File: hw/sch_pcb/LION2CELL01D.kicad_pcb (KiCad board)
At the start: 2 copper layers, 80.8 x 60.5 mm, 100 parts, among them J1 JUMP_4X2, J10 JUMP_2x1, J11 JUMP_2x1, J12 JUMP_2x1, J13 JUMP_4X2, J14 JUMP_2x1, J15 CONN_2, J2 JUMP_2x1, J3 JUMP_2x1, J4 JUMP2_2x1, J5 JUMP_2x1, J6 JUMP_2x1, J7 JUMP_4X2, J8 CONN1_1, J9 CONN1_1, P1 _, P2 _, P3 _, P4 _, Q1 IRLML6244, SW1 SW_PUSH, U1 BQ29209, U2 BQ24103, U3 BQ34Z100, U4 SN74HC164D, U5 TPS76601, U6 APX810-31SAG-7

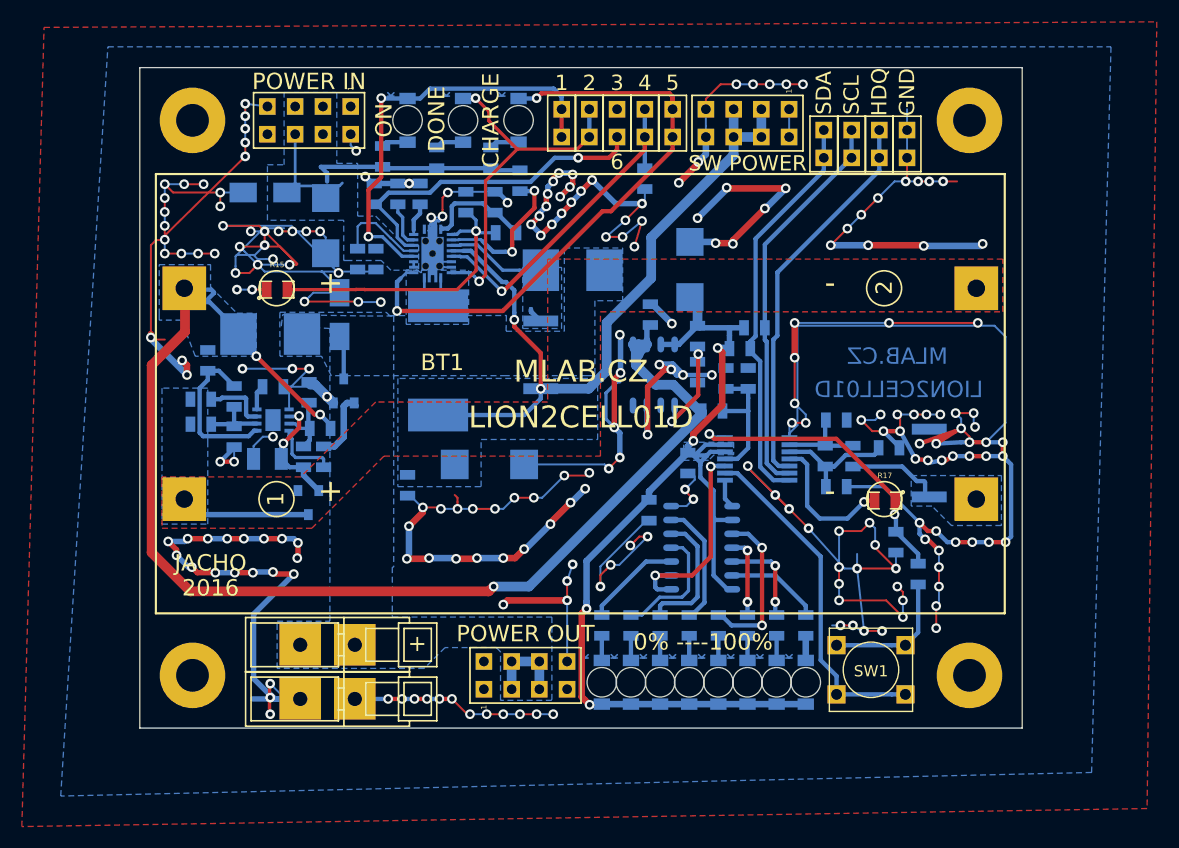
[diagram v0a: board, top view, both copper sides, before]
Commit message: Documentation update.
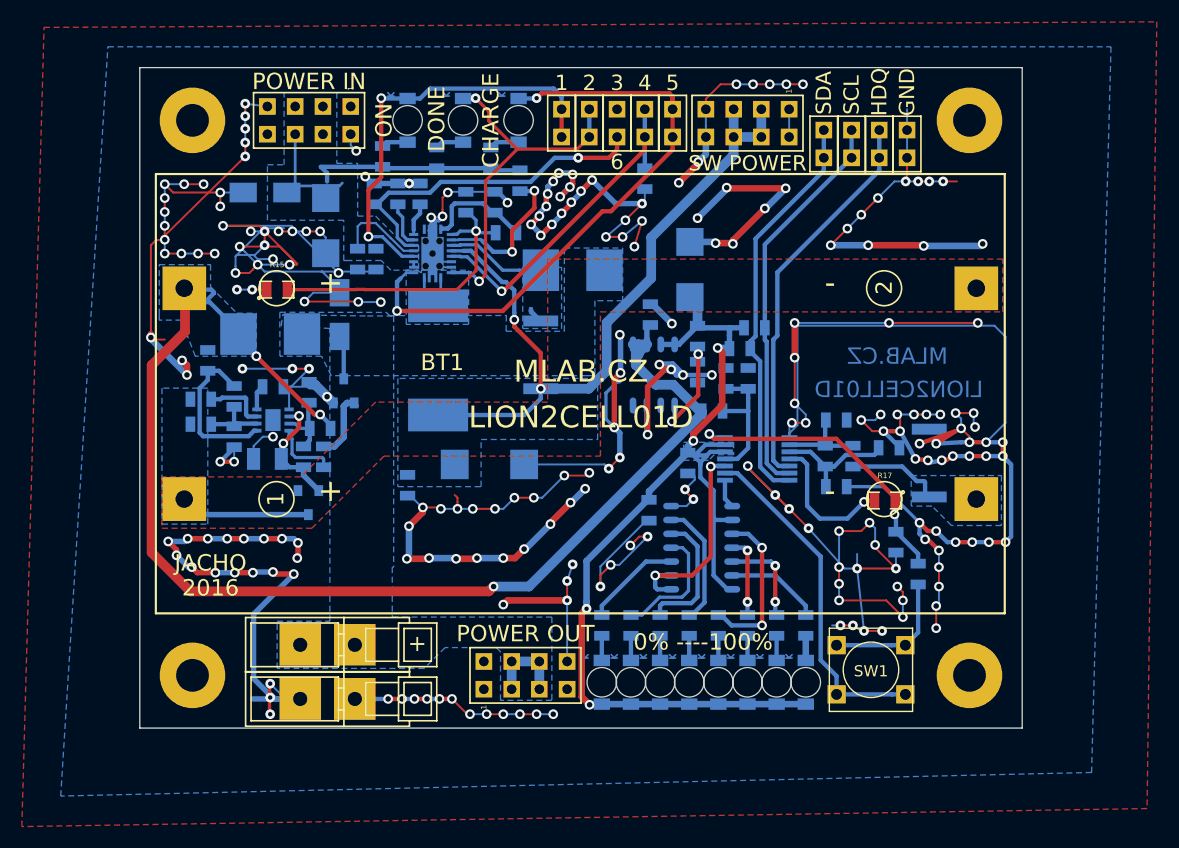
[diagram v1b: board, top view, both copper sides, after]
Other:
- net class Default removed
- net class Low_power removed
